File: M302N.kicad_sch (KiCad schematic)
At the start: 29 parts, among them J1 DC12V, J10 ADC_IN, J11 RJ45, J12 DC12V FAN, J2 UART, J3 extend I/O, J4 I2C-1, J5 ADC_IN, J6 ADC_IN, J7 ADC_IN, J8 ADC_IN, J9 ADC_IN, SW1 SW_Reed, U1 W5500, U2 NJM2845DL1-05

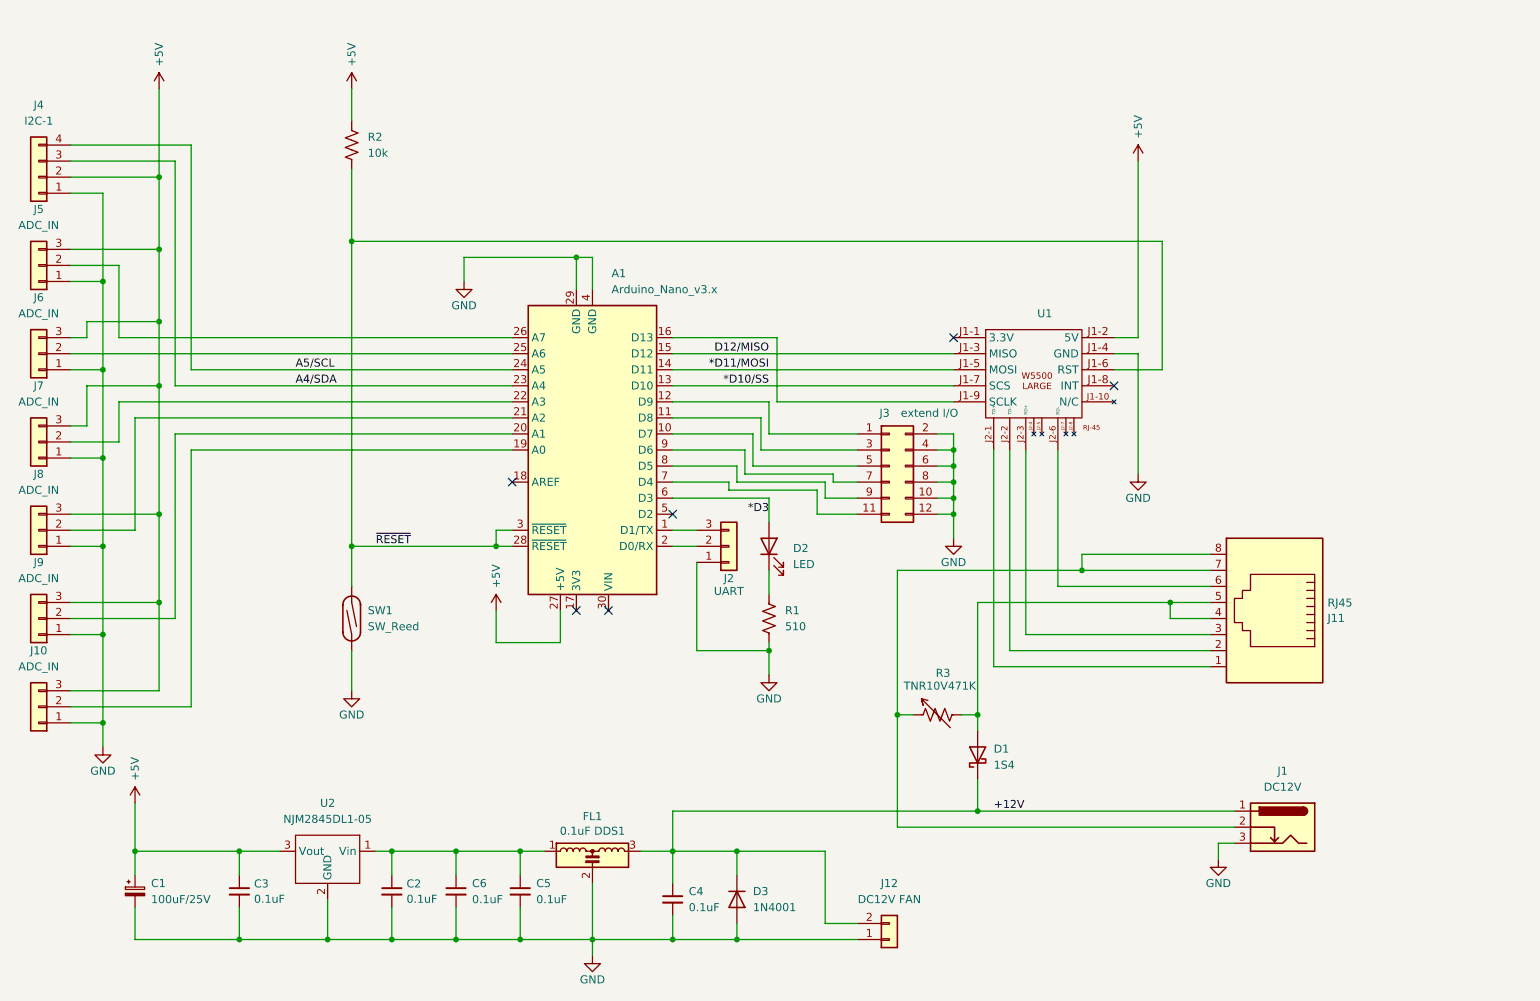
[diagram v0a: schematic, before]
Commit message: PCB設計途中
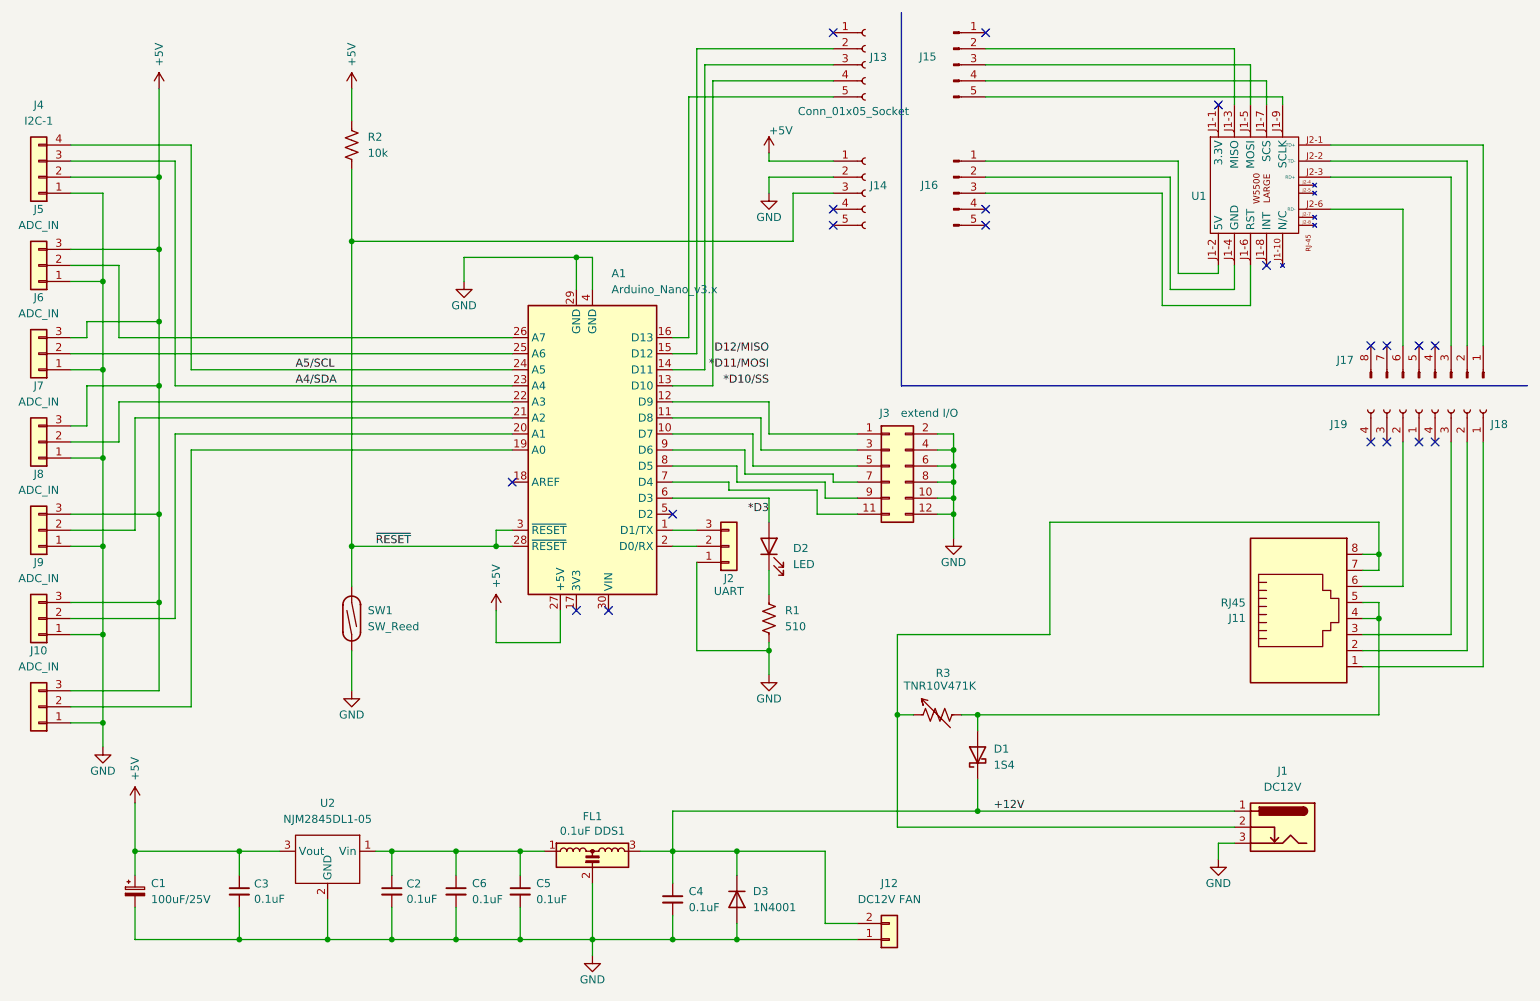
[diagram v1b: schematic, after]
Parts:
- added J13, J14: Conn_01x05_Socket, Connector_PinSocket_2.54mm:PinSocket_1x05_P2.54mm_Vertical, symbol Connector:Conn_01x05_Socket
- added J15, J16: Conn_01x05_Pin, symbol Connector:Conn_01x05_Pin
- added J17: Conn_01x08_Pin, symbol Connector:Conn_01x08_Pin
- added J18, J19: Conn_01x04_Socket, Connector_PinSocket_2.54mm:PinSocket_1x04_P2.54mm_Vertical, symbol Connector:Conn_01x04_Socket
- A1: footprint Arduino:Arduino_Nano -> Module:Arduino_Nano
- SW1: footprint (none) -> HOLLY:REED_SW
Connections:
- net *D10/SS: no longer A1.13 (D10), U1.J1-7 (SCS)
- net *D11/MOSI: no longer A1.14 (D11), U1.J1-5 (MOSI)
- net +5V: now also J14.1 (Pin_1); no longer U1.J1-2 (5V)
- net D12/MISO: no longer A1.15 (D12), U1.J1-3 (MISO)
- net GND: now also J14.2 (Pin_2); no longer U1.J1-4 (GND)
- net ~{RESET}: now also J14.3 (Pin_3); no longer U1.J1-6 (RST)
- net at U1.J2-1 (TD+): now also J17.1 (Pin_1); no longer J11.1
- net at U1.J2-2 (TD-): now also J17.2 (Pin_2); no longer J11.2
- net at U1.J2-3 (RD+): now also J17.3 (Pin_3); no longer J11.3
- net at U1.J2-6 (RD-): now also J17.6 (Pin_6); no longer J11.6
- net at A1.16 (D13): now also J13.5 (Pin_5); no longer U1.J1-9 (SCLK)
- new net: A1.15 (D12), J13.2 (Pin_2)
- new net: A1.14 (D11), J13.3 (Pin_3)
- new net: A1.13 (D10), J13.4 (Pin_4)
- new net: J16.1 (Pin_1), U1.J1-2 (5V)
- new net: J16.2 (Pin_2), U1.J1-4 (GND)
- new net: J16.3 (Pin_3), U1.J1-6 (RST)
- new net: J11.6, J19.2 (Pin_2)
- new net: J11.1, J18.1 (Pin_1)
- new net: J11.2, J18.2 (Pin_2)
- new net: J11.3, J18.3 (Pin_3)
- new net: J15.2 (Pin_2), U1.J1-3 (MISO)
- new net: J15.3 (Pin_3), U1.J1-5 (MOSI)
- new net: J15.4 (Pin_4), U1.J1-7 (SCS)
- new net: J15.5 (Pin_5), U1.J1-9 (SCLK)
- no-connect marks 6 -> 20
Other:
- moved on the sheet: J11, U1
